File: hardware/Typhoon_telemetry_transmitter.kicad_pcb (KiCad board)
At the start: 2 copper layers, 44.7 x 34.1 mm, 24 parts, among them J1 Conn_01x04_Pin, J3 Conn_ST_STDC14, SW1 SW_Push, U1 STM32F103C8Tx, U2 NRF24L01_Breakout, Y1 8M

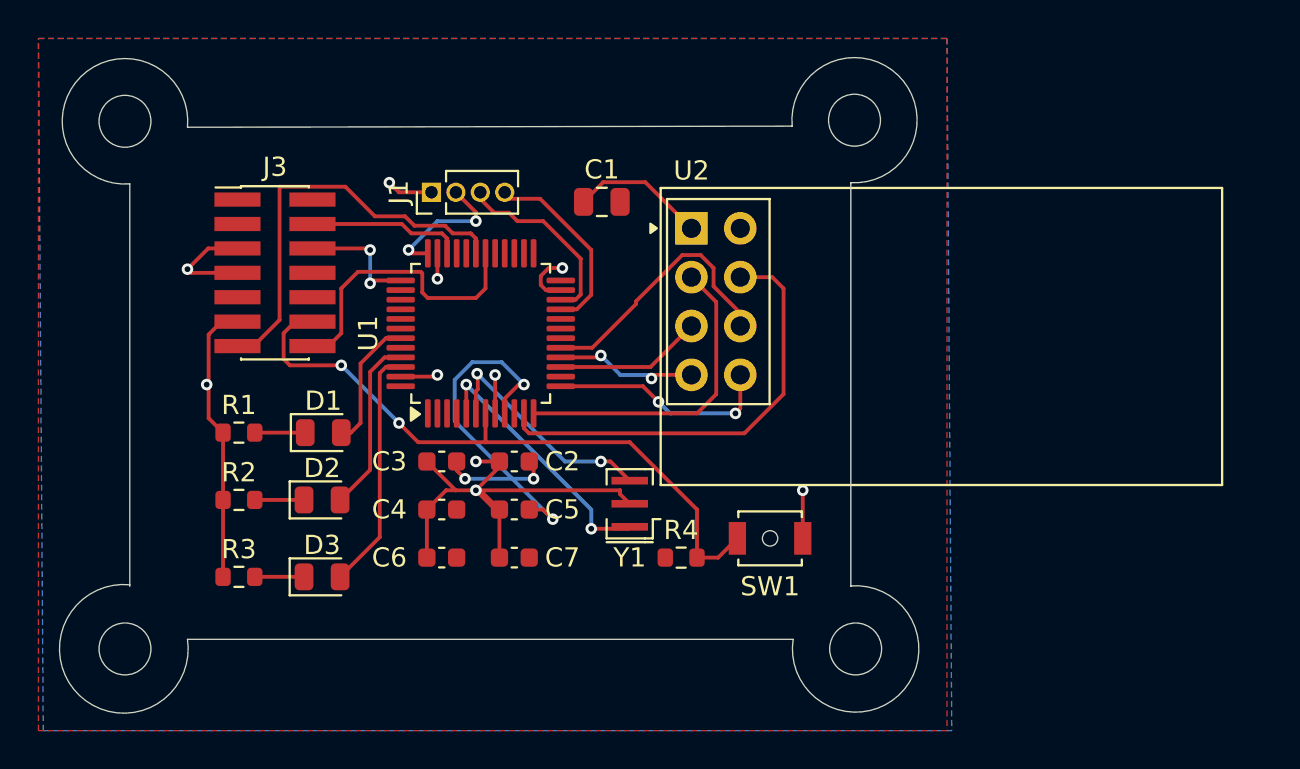
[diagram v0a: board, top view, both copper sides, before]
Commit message: Final Update
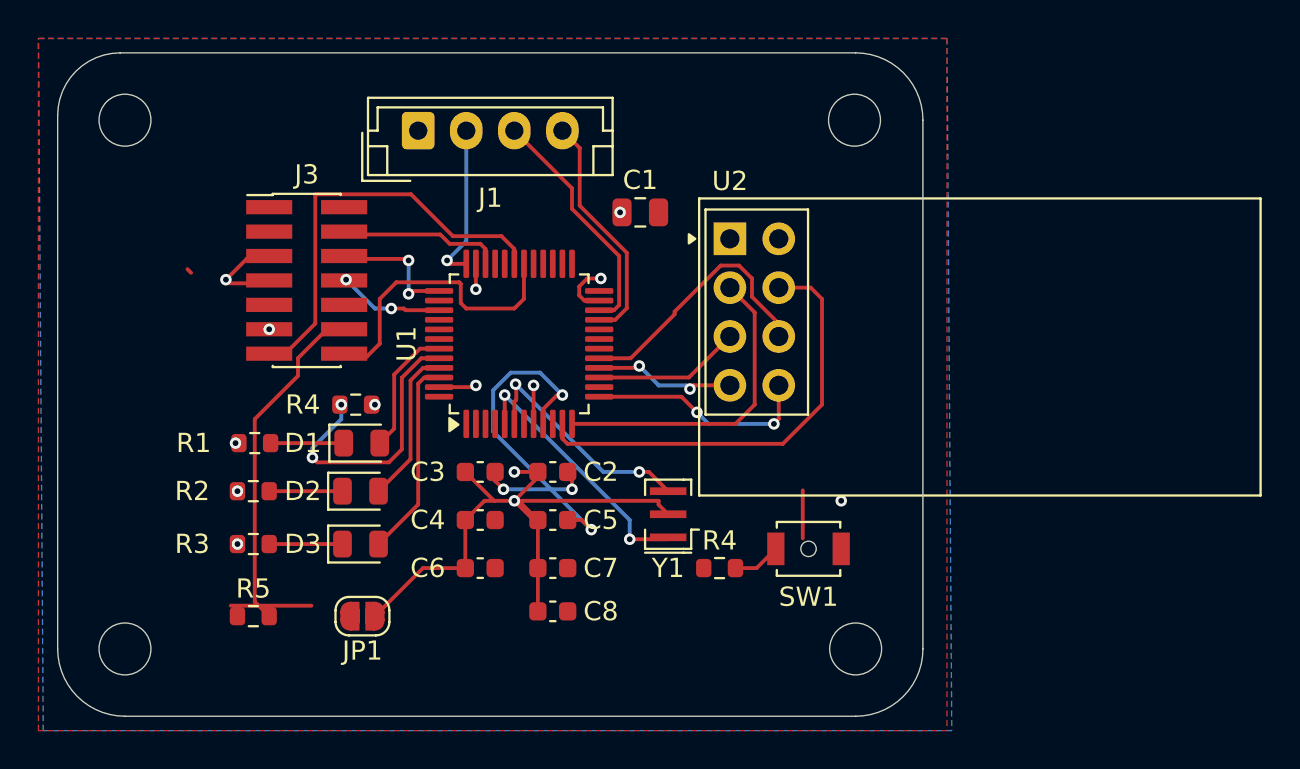
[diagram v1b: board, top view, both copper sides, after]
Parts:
- added C8: 0.1u, Capacitor_SMD:C_0603_1608Metric, F.Cu at (155.0, 91.8)
- added JP1: Jumper_2_Open, Jumper:SolderJumper-2_P1.3mm_Open_RoundedPad1.0x1.5mm, F.Cu at (145.1, 92.0)
- added R4: 10k, Resistor_SMD:R_0603_1608Metric, F.Cu at (144.8, 81.0)
- added R5: 10k, Resistor_SMD:R_0603_1608Metric, F.Cu at (139.4, 92.0)
- J1: footprint Connector_PinHeader_1.27mm:PinHeader_1x04_P1.27mm_Vertical -> Connector_JST:JST_EH_B4B-EH-A_1x04_P2.50mm_Vertical
- moved J1 3.28 mm to (148.0, 66.8), turned to 0 degrees
- moved D3 2.63 mm to (145.0, 88.3)
- moved C1 2.07 mm to (159.6, 71.0)
- moved C2 2.07 mm to (155.0, 84.5)
- moved C3 2.07 mm to (151.2, 84.5)
- moved C4 2.07 mm to (151.2, 87.0)
- moved C5 2.07 mm to (155.0, 87.0)
- moved C6 2.07 mm to (151.2, 89.5)
- moved C7 2.07 mm to (155.0, 89.5)
- moved D1 2.07 mm to (145.1, 83.0)
- moved R4 2.07 mm to (163.7, 89.5)
- moved SW1 2.07 mm to (168.3, 88.5)
- moved U2 2.07 mm to (164.2, 72.4)
- moved Y1 2.07 mm to (161.0, 86.7)
- moved U1 2.07 mm to (153.2, 77.9)
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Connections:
- net /Programming_RX renamed /STLINK_{RX}
- net /Programming_TX renamed /STLINK_{TX}
- net /codeclk renamed /SWCLK
- net /codeio renamed /SWDIO
- J3 pad 12: /Reset -> Net-(J3-~{RST})
- J3 pad 8: unconnected-(J3-JTDO/SWO-Pad8) -> /SWO
- U1 pad 39: unconnected-(U1-PB3-Pad39) -> /SWO
- U1 pad 44: unconnected-(U1-BOOT0-Pad44) -> Net-(U1-BOOT0)
- U1 pad 7: /Reset -> unconnected-(U1-NRST-Pad7)
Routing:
- net /Reset: track 34.3 -> 2.51 mm, vias 2 -> 0
- net Net-(J3-~{RST}): track 0.00 -> 21.9 mm
- net GND: track 65.5 -> 49.4 mm, vias 10 -> 14
- net Net-(U1-BOOT0): track 0.00 -> 14.5 mm, vias 0 -> 2
- net /SWO: track 0.00 -> 5.50 mm, vias 0 -> 2
- net /RX: track 9.52 -> 12.5 mm
- net Net-(D3-A): track 12.7 -> 10.4 mm
- net /TX: track 10.1 -> 12.3 mm
- net Net-(D3-K): track 2.56 -> 3.81 mm
- net Net-(D2-K): track 2.56 -> 3.81 mm
- net Net-(D1-K): track 2.62 -> 3.80 mm
- net +3.3V: track 30.1 -> 31.2 mm, vias 6 -> 5
- net Net-(D2-A): track 9.21 -> 8.21 mm
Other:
- board size 44.7 x 34.1 mm -> 45 x 34.5 mm

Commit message: Final Final Updates
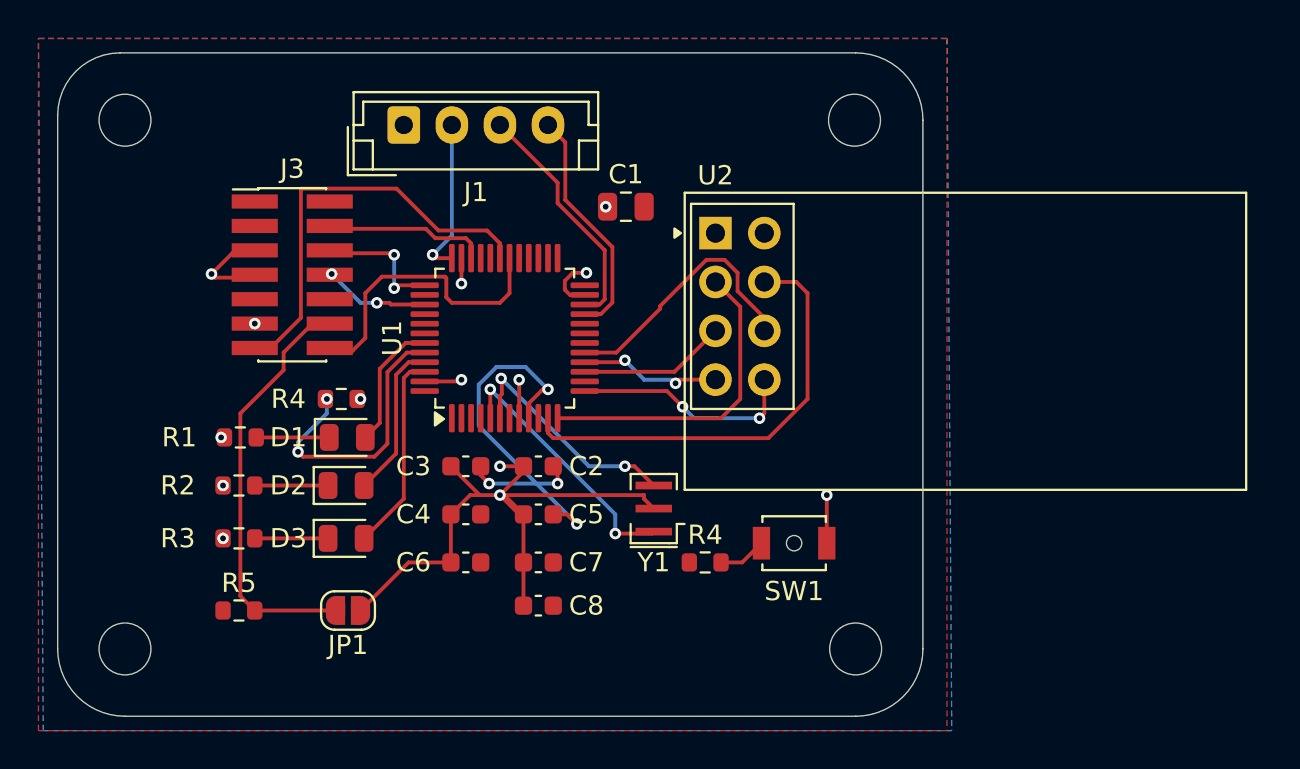
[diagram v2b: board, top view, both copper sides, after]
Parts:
- moved C1 0.81 mm to (158.8, 70.8)
- moved C2 0.81 mm to (154.2, 84.2)
- moved C3 0.81 mm to (150.5, 84.2)
- moved C4 0.81 mm to (150.5, 86.8)
- moved C5 0.81 mm to (154.2, 86.8)
- moved C6 0.81 mm to (150.5, 89.2)
- moved C7 0.81 mm to (154.2, 89.2)
- moved C8 0.81 mm to (154.2, 91.5)
- moved D1 0.81 mm to (144.3, 82.8)
- moved D2 0.81 mm to (144.2, 85.2)
- moved D3 0.81 mm to (144.2, 88.0)
- moved J1 0.81 mm to (147.2, 66.5)
- moved JP1 0.81 mm to (144.3, 91.8)
- moved R1 0.81 mm to (138.8, 82.8)
- moved R2 0.81 mm to (138.7, 85.2)
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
